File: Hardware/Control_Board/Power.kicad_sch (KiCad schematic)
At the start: 2 parts, among them U2 TPS62933, U4 LT1963AxST-3.3

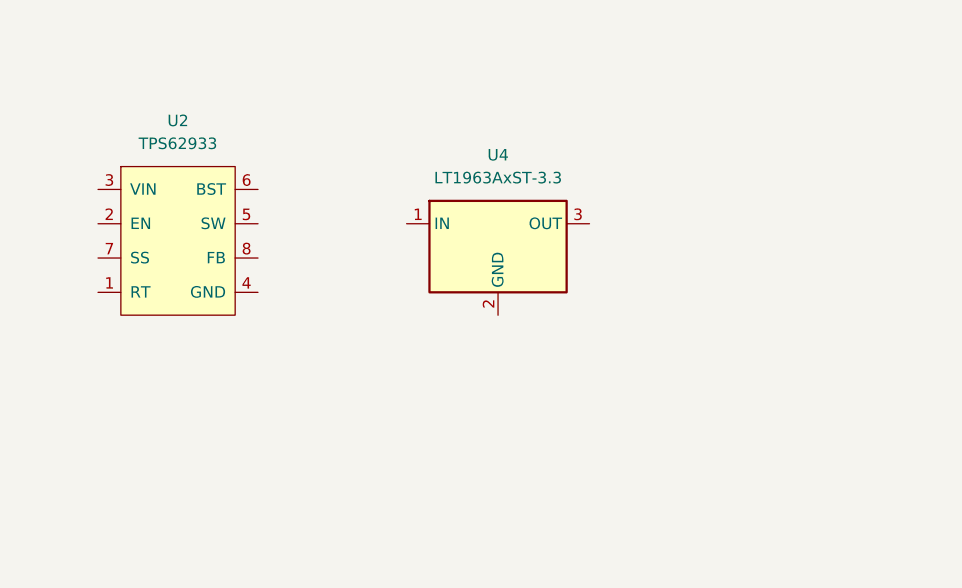
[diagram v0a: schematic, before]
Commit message: fleshed out info/planning, roughed in more schematics, added short readme
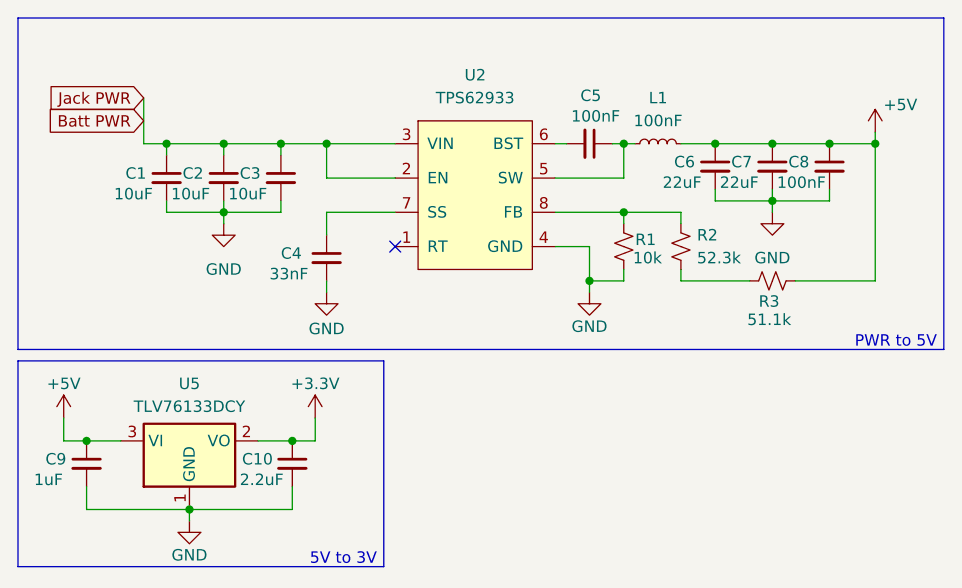
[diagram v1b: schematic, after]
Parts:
- removed U4: LT1963AxST-3.3, Package_TO_SOT_SMD:SOT-223-3_TabPin2, symbol Regulator_Linear:LT1963AxST-3.3
- added C1, C2, C3: 10uF, Capacitor_SMD:C_0805_2012Metric_Pad1.18x1.45mm_HandSolder, symbol Device:C_Small
- added C10: 2.2uF, Capacitor_SMD:C_0805_2012Metric_Pad1.18x1.45mm_HandSolder, symbol Device:C_Small
- added C4: 33nF, Capacitor_SMD:C_0603_1608Metric_Pad1.08x0.95mm_HandSolder, symbol Device:C_Small
- added C5: 100nF, Capacitor_SMD:C_0603_1608Metric_Pad1.08x0.95mm_HandSolder, symbol Device:C_Small
- added C6, C7: 22uF, Capacitor_SMD:C_0805_2012Metric_Pad1.18x1.45mm_HandSolder, symbol Device:C_Small
- added C8: 100nF, Capacitor_SMD:C_0201_0603Metric_Pad0.64x0.40mm_HandSolder, symbol Device:C_Small
- added C9: 1uF, Capacitor_SMD:C_0805_2012Metric_Pad1.18x1.45mm_HandSolder, symbol Device:C_Small
- added L1: 100nF, symbol Device:L_Small
- added R1: 10k, Resistor_SMD:R_0603_1608Metric_Pad0.98x0.95mm_HandSolder, symbol Device:R_Small_US
- added R2: 52.3k, Resistor_SMD:R_0603_1608Metric_Pad0.98x0.95mm_HandSolder, symbol Device:R_Small_US
- added R3: 51.1k, Resistor_SMD:R_0603_1608Metric_Pad0.98x0.95mm_HandSolder, symbol Device:R_Small_US
- added U5: TLV76133DCY, Package_TO_SOT_SMD:SOT-223-3_TabPin2, symbol Regulator_Linear:TLV76133DCY
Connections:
- net Batt PWR: now reaches U2.2 (EN)
- net Batt PWR: now also U2.3 (VIN), C1.1, C2.1, C3.1
- net GND: now reaches U2.4 (GND)
- net GND: now also C1.2, C10.2, C2.2, C3.2, C4.2, C6.2, C7.2, C8.2, C9.2, R1.2, U5.1 (GND)
- net at U2.5 (SW): now also C5.1, L1.1
- net at U2.6 (BST): now also C5.2
- net at U2.7 (SS): now also C4.1
- net at U2.8 (FB): now also R1.1, R2.1
- new net: R2.2, R3.2
- new net +3.3V: C10.1, U5.2 (VO)
- new net +5V: C6.1, C7.1, C8.1, C9.1, L1.2, R3.1, U5.3 (VI)
- no-connect marks 0 -> 1
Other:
- note added: "5V to 3V"
- note added: "PWR to 5V"
- moved on the sheet: U2
